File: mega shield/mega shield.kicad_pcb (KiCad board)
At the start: 2 copper layers, 30 parts, among them J1 Conn_01x08_Male, J10 Conn_01x04_Male, J11 Conn_01x04_Male, J12 Conn_01x04_Male, J13 Conn_01x03_Male, J14 Conn_01x03_Male, J15 Conn_01x03_Male, J16 Conn_01x03_Male, J17 POWER IN, J18 3.3V OUT, J2 Conn_01x08_Male, J3 Conn_01x08_Male, J4 Conn_01x08_Male, J5 Conn_01x08_Male, J6 Conn_01x08_Male, J7 Conn_01x04_Male, J8 Conn_01x04_Male, J9 Conn_01x04_Male, SW1 RST

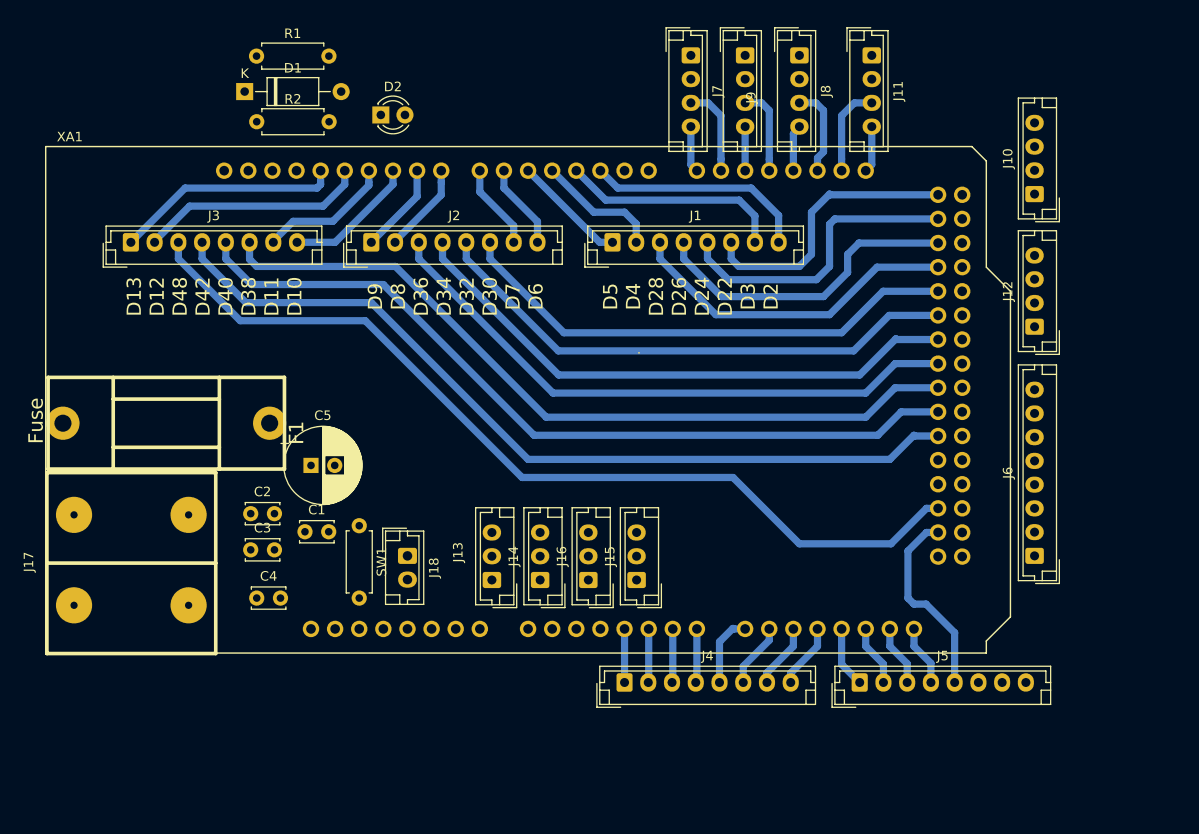
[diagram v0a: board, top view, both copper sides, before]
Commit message: mega shield completed
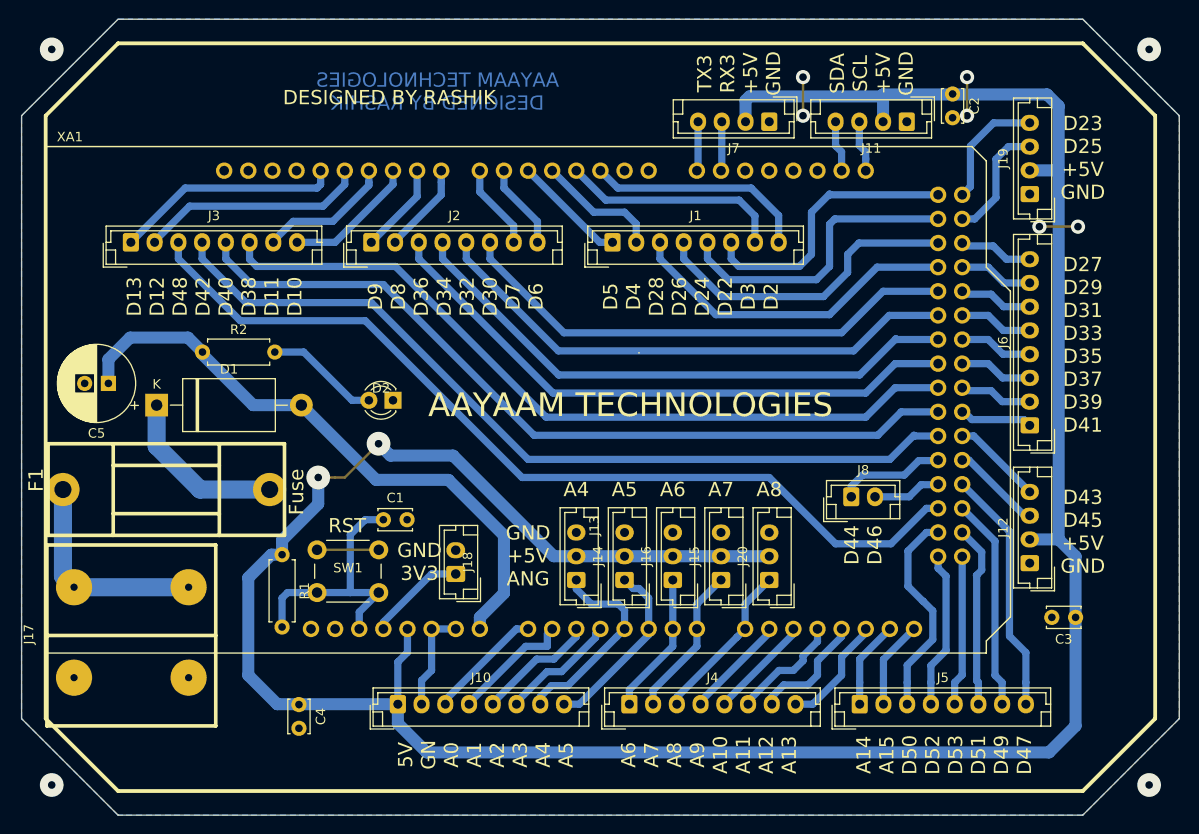
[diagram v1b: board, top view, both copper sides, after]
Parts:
- removed J9: Conn_01x04_Male, Connector_JST:JST_EH_B4B-EH-A_1x04_P2.50mm_Vertical
- added J19: Conn_01x04_Male, Connector_JST:JST_EH_B4B-EH-A_1x04_P2.50mm_Vertical, F.Cu at (192.5, 66.7)
- added J20: Conn_01x03_Male, Connector_JST:JST_EH_B3B-EH-A_1x03_P2.50mm_Vertical, F.Cu at (165.1, 107.3)
- D1: footprint Diode_THT:D_A-405_P10.16mm_Horizontal -> Diode_THT:D_DO-27_P15.24mm_Horizontal
- J10: value Conn_01x04_Male -> Conn_01x08_Male; footprint Connector_JST:JST_EH_B4B-EH-A_1x04_P2.50mm_Vertical -> Connector_JST:JST_EH_B8B-EH-A_1x08_P2.50mm_Vertical
- J8: value Conn_01x04_Male -> Conn_01x02_Male; footprint Connector_JST:JST_EH_B4B-EH-A_1x04_P2.50mm_Vertical -> Connector_JST:JST_EH_B2B-EH-A_1x02_P2.50mm_Vertical
- SW1: footprint Resistor_THT:R_Axial_DIN0207_L6.3mm_D2.5mm_P7.62mm_Horizontal -> Button_Switch_THT:SW_PUSH_6mm_H5mm
- moved C3 87.2 mm to (197.4, 111.3), turned to 180 degrees
- moved C2 86.1 mm to (184.4, 56.1), turned to 270 degrees
- moved J10 85.9 mm to (126.0, 120.4), turned to 0 degrees
- moved R1 52.6 mm to (113.8, 104.6), turned to 270 degrees
- moved J8 46.8 mm to (173.7, 98.6), turned to 0 degrees
- moved D1 34.3 mm to (100.6, 88.9)
- moved D2 30.1 mm to (125.5, 88.4), turned to 180 degrees
- moved R2 24.9 mm to (105.4, 83.3)
- moved J12 24.9 mm to (192.5, 105.5)
- moved C5 23.0 mm to (95.5, 86.6), turned to 180 degrees
- moved J6 13.8 mm to (192.5, 91.0)
- moved C4 12.1 mm to (115.6, 120.4), turned to 270 degrees
- moved J7 10.8 mm to (165.1, 59.1), turned to 180 degrees
- moved J13 8.89 mm to (144.8, 107.3)
- moved J14 8.89 mm to (149.9, 107.3)
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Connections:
- J10 pad 1: D27 -> +5V
- J10 pad 2: D29 -> GND
- J10 pad 3: +5V -> A0
- J10 pad 4: GND -> A1
- J11 pad 3: SDA -> SCL
- J11 pad 4: SCL -> SDA
- J12 pad 1: D23 -> GND
- J12 pad 2: D25 -> +5V
- J12 pad 3: +5V -> D45
- J12 pad 4: GND -> D43
- J13 pad 1: A0 -> A4
- J14 pad 1: A1 -> A5
- J15 pad 1: A3 -> A7
- J16 pad 1: A2 -> A6
- J18 pad 1: GND -> +3V3
- J18 pad 2: +3V3 -> GND
- J4 pad 1: A4 -> A6
- J4 pad 2: A5 -> A7
- J4 pad 3: A6 -> A8
- J4 pad 4: A7 -> A9
- J4 pad 5: A8 -> A10
- J4 pad 6: A9 -> A11
- J4 pad 7: A10 -> A12
- J4 pad 8: A11 -> A13
- J5 pad 1: A12 -> A14
- J5 pad 2: A13 -> A15
- J5 pad 3: A14 -> D50
- J5 pad 4: A15 -> D52
- J5 pad 5: D50 -> D53
- J6 pad 1: D45 -> D41
- J6 pad 2: D43 -> D39
- J6 pad 3: D41 -> D37
- J6 pad 4: D39 -> D35
- J6 pad 5: D37 -> D33
- J6 pad 6: D35 -> D31
- J6 pad 7: D33 -> D29
- J6 pad 8: D31 -> D27
- J8 pad 1: GND -> D44
- J8 pad 2: +5V -> D46
- R1 pad 1: Net-(R1-Pad1) -> +5V
- XA1 pad GND1: Net-(XA1-PadGND1) -> GND
- XA1 pad GND2: Net-(XA1-PadGND1) -> GND
- XA1 pad GND3: Net-(XA1-PadGND1) -> GND
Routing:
- net +5V: track 0.00 -> 290.6 mm, vias 0 -> 2
- net +12V: track 0.00 -> 64.8 mm
- net GND: track 0.00 -> 29.6 mm, vias 0 -> 6
- net Net-(C1-Pad1): track 0.00 -> 28.4 mm
- net D47: track 0.00 -> 25.9 mm
- net Net-(F1-Pad2): track 0.00 -> 22.8 mm
- net D49: track 0.00 -> 22.4 mm
- net D51: track 0.00 -> 19.3 mm
- net Net-(D1-Pad1): track 0.00 -> 18.1 mm
- net D52: track 0.00 -> 16.6 mm
- net A4: track 5.64 -> 21.5 mm
- net D53: track 0.00 -> 15.9 mm
- net A5: track 5.66 -> 19.1 mm
- net A1: track 0.00 -> 12.9 mm
- net D23: track 0.00 -> 12.7 mm
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- added copper zone on B.Cu, net GND
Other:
- board outline added: 121.9 x 83.8 mm
- board text added: "5V GN A0 A1 A2 A3 A4 A5"
- board text added: "A14 A15 D50 D52 D53 D51 D49 D47"
- board text added: "A4"
- board text added: "A5"
- board text added: "A6"
- board text added: "A6 A7 A8 A9 A10 A11 A12 A13"
- board text added: "A7"
- board text added: "A8"
- board text added: "AAYAAM TECHNOLOGIES"
- board text added: "AAYAAM TECHNOLOGIES DESIGNED BY RASHIK"
- board text added: "D23 D25 +5V GND"
- board text added: "D27 D29 D31 D33 D35 D37 D39 D41"
- board text added: "D43 D45 +5V GND"
- board text added: "D44 D46"
- board text added: "DESIGNED BY RASHIK"
- board text added: "GND +5V ANG"
- board text added: "GND 3V3"
- board text added: "RST"
- board text added: "SDA SCL +5V GND"
- board text added: "TX3 RX3 +5V GND"
